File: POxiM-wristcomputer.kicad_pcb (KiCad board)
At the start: 4 copper layers, 40 x 23.5 mm, 82 parts, among them J1 USB_B_Micro, J14 Jumper_NO_Small, J2 AudioJack4_Ground

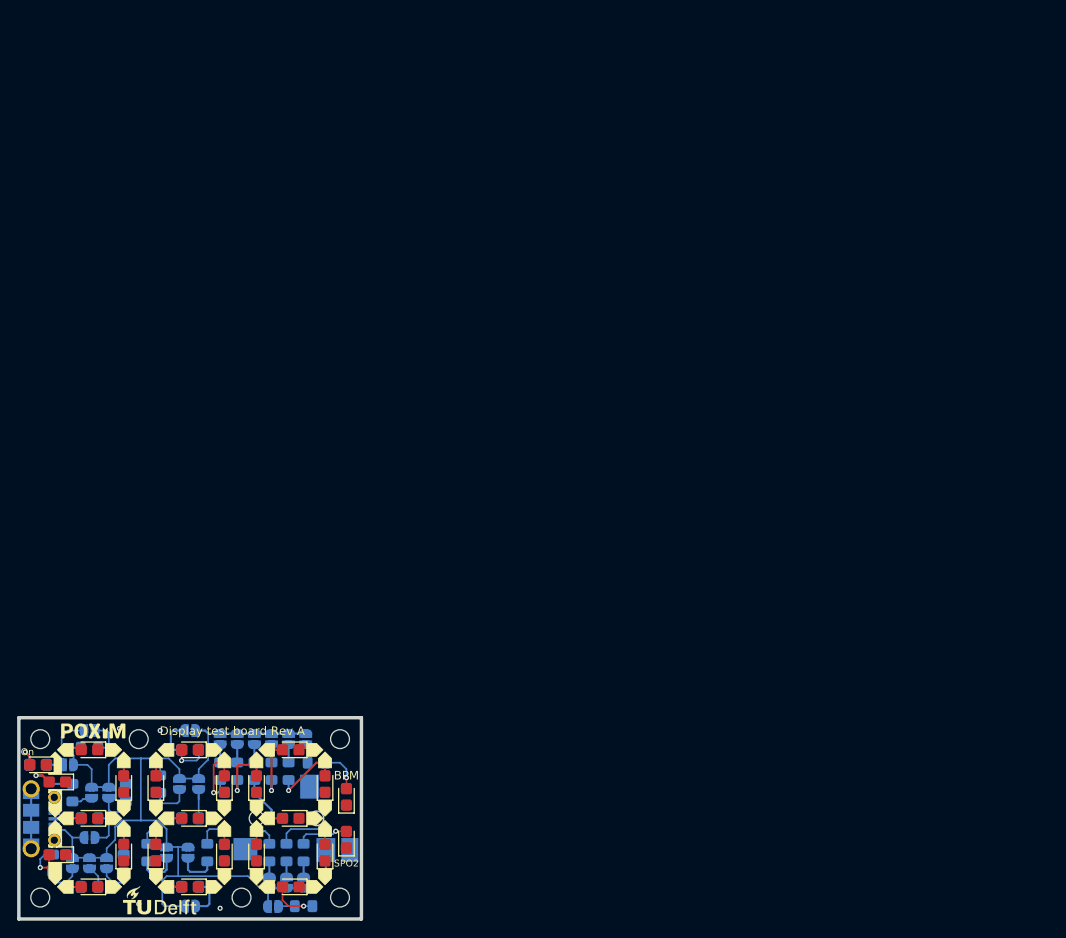
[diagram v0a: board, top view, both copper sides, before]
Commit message: Finish works-as prototype design
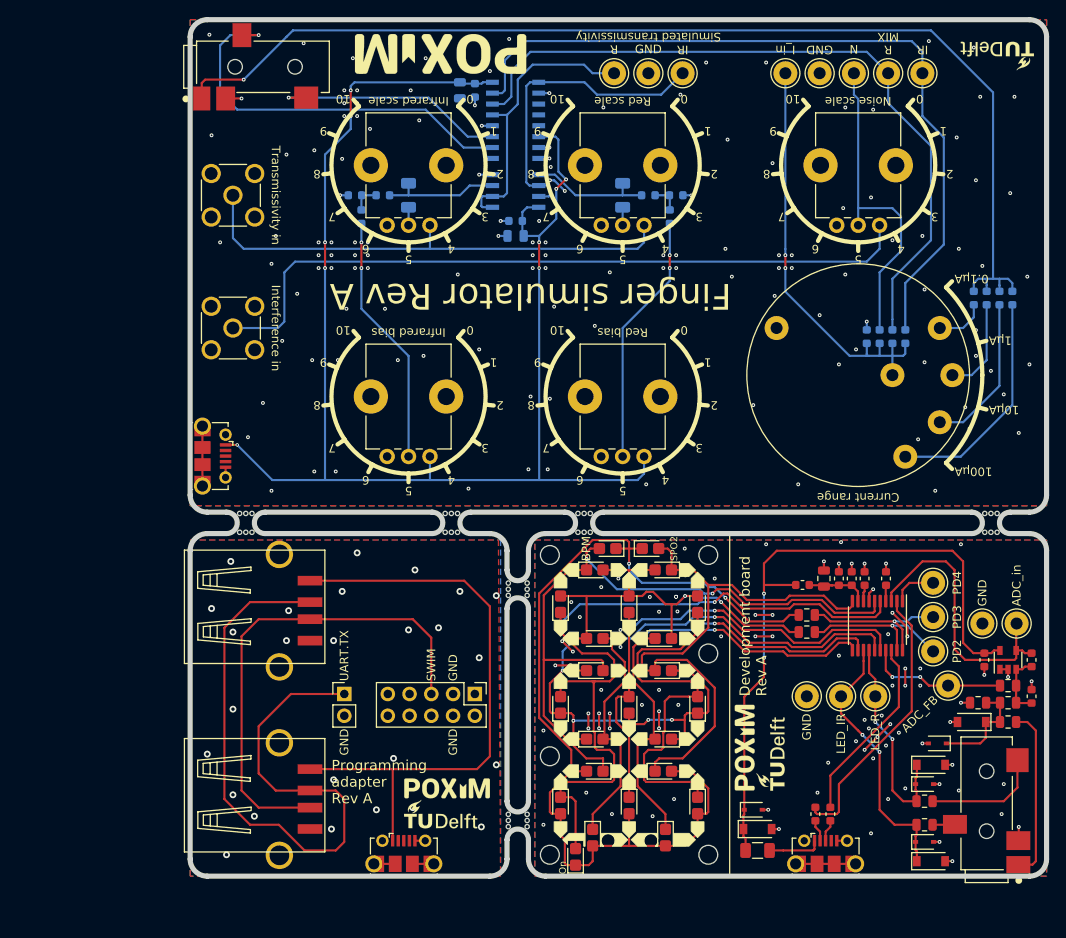
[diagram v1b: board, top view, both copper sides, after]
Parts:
- removed the G*** at (86.4, 142.8)
- removed the G*** at (78.7, 123.0)
- removed J14, JP16, JP18, JP20, JP27, JP28, JP29, JP30, JP31, JP8: Jumper_NO_Small, POxiM-uncategorised:SolderJumper-2_P1.3mm_Open_RoundedPad1.0x1.5mm
- removed JP10, JP11, JP12, JP13, JP15, JP17, JP19, JP21, JP22, JP23, JP24, JP25, JP26, JP9: Jumper_NC_Small, POxiM-uncategorised:SolderJumper-2_P1.3mm_SolderBridged_RoundedPad1.0x1.5mm
- removed R20, R21, R22, R23, R24, R25, R26, R27, R28, R29, R30: 4.7kΩ, Resistor_SMD:R_0805_2012Metric_Pad1.15x1.40mm_HandSolder
- added C1: 100nF, Capacitor_SMD:C_0603_1608Metric, F.Cu at (182.7, 114.8)
- added C10: 2.2uF, Capacitor_SMD:C_0805_2012Metric, B.Cu at (128.0, 65.2)
- added C11: 100nF, Capacitor_SMD:C_0603_1608Metric, B.Cu at (128.0, 63.5)
- added C12: 100nF, Capacitor_SMD:C_0603_1608Metric, B.Cu at (123.2, 48.2)
- added C13: 2.2uF, Capacitor_SMD:C_0805_2012Metric, B.Cu at (121.5, 48.2)
- added C14: 6.8uF, Capacitor_SMD:C_1206_3216Metric, B.Cu at (115.5, 60.5)
- added C15: 6.8uF, Capacitor_SMD:C_1206_3216Metric, B.Cu at (140.5, 60.5)
- added C16: 100nF, Capacitor_SMD:C_0603_1608Metric, B.Cu at (109.2, 60.5)
- added C17: 100nF, Capacitor_SMD:C_0603_1608Metric, B.Cu at (146.8, 60.5)
- added C2: 100pF, Capacitor_SMD:C_0603_1608Metric, F.Cu at (188.2, 114.8)
- added C3: 100nF, Capacitor_SMD:C_0603_1608Metric, F.Cu at (188.2, 119.0)
- added C4: 2.2uF, Capacitor_SMD:C_0805_2012Metric, F.Cu at (182.0, 119.8)
- added C5: 100nF, Capacitor_SMD:C_0603_1608Metric, F.Cu at (171.2, 105.2)
- added C6: 2.2uF, Capacitor_SMD:C_0805_2012Metric, F.Cu at (164.0, 105.2)
- added C7: 470nF, Capacitor_SMD:C_0603_1608Metric, F.Cu at (168.8, 105.2)
- added C8: 100nF, Capacitor_SMD:C_0603_1608Metric, F.Cu at (165.8, 105.2)
- added C9: 100nF, Capacitor_SMD:C_0603_1608Metric, F.Cu at (167.2, 105.2)
- added D1: 5.2V, Diode_SMD:D_SOD-123, F.Cu at (176.5, 138.2)
- added D2: ~, Diode_SMD:D_SOD-323, F.Cu at (175.8, 136.0)
- added D3: 5.2V, Diode_SMD:D_SOD-123, F.Cu at (176.5, 127.0)
- added D31: 5.2V, Diode_SMD:D_SOD-123, F.Cu at (156.2, 134.5)
- added D32: ~, Diode_SMD:D_SOD-323, F.Cu at (155.8, 132.2)
- added D4: ~, Diode_SMD:D_SOD-323, F.Cu at (175.8, 129.2)
- added D5: 5.2V, Diode_SMD:D_SOD-123, F.Cu at (181.2, 122.0)
- added D6: ~, Diode_SMD:D_SOD-323, F.Cu at (177.2, 124.5)
- added F1: 100mA, Resistor_SMD:R_1206_3216Metric, F.Cu at (156.2, 137.0)
- added FB1: Ferrite_Bead_Small, Inductor_SMD:L_0603_1608Metric, F.Cu at (161.5, 106.0)
- added G***: LOGO, POxiM-logos:POxiMLogo_GoldHeart_W10mm, F.Cu at (120.0, 129.8)
- added G***: LOGO, POxiM-logos:TUDelftLogo_W10mm, F.Cu at (119.2, 132.8)
- added G***: LOGO, POxiM-logos:TUDelftLogo_W10mm, F.Cu at (157.8, 125.8)
- added G***: LOGO, POxiM-logos:POxiMLogo_GoldHeart_W10mm, F.Cu at (154.8, 125.0)
- added G***: LOGO, POxiM-logos:TUDelftLogo_W10mm, F.Cu at (184.2, 44.2)
- added G***: LOGO, POxiM-logos:POxiMLogo_GoldHeart_W20mm, F.Cu at (119.2, 44.0)
- added J10: Transmissivity in, Connector_Coaxial:SMA_Molex_73251-2200_Horizontal, F.Cu at (95.0, 60.5)
- added J11: AudioJack4_Ground, POxiM-uncategorised:CUI_SJ-43514-SMT, F.Cu at (98.5, 45.5)
- added J3: USB_B_Micro, POxiM-uncategorised:Micro-B_Molex_105017-0001, F.Cu at (115.0, 140.0)
- added J4: USB_A, POxiM-uncategorised:USBA_87583-2010RLF, F.Cu at (104.0, 131.0)
- added J5: USB_A, POxiM-uncategorised:USBA_87583-2010RLF, F.Cu at (104.0, 109.0)
- added J6: Uart Out, Connector_PinHeader_2.54mm:PinHeader_1x02_P2.54mm_Vertical, F.Cu at (108.0, 118.7)
- added J7: Programming Header, Connector_PinHeader_2.54mm:PinHeader_2x05_P2.54mm_Vertical, F.Cu at (123.2, 118.7)
- added J8: USB_B_Micro, POxiM-uncategorised:Micro-B_Molex_105017-0001, F.Cu at (90.0, 91.0)
- added J9: Interference in, Connector_Coaxial:SMA_Molex_73251-2200_Horizontal, F.Cu at (95.0, 76.0)
- added JP1: Jumper_2_Open, Resistor_SMD:R_0603_1608Metric, F.Cu at (164.8, 132.8)
- added JP2: Jumper_2_Open, Resistor_SMD:R_0603_1608Metric, F.Cu at (163.0, 132.8)
- added MB1: Bumpon, POxiM-uncategorised:Bumpon-SJ-5007BK, B.Cu at (96.0, 131.0)
- added MB10: Bumpon, POxiM-uncategorised:Bumpon-SJ-5007BK, B.Cu at (184.0, 46.0)
- added MB11: Bumpon, POxiM-uncategorised:Bumpon-SJ-5007BK, B.Cu at (184.0, 91.5)
- added MB12: Bumpon, POxiM-uncategorised:Bumpon-SJ-5007BK, B.Cu at (96.0, 91.5)
- added MB2: Bumpon, POxiM-uncategorised:Bumpon-SJ-5007BK, B.Cu at (96.0, 109.0)
- added MB3: Bumpon, POxiM-uncategorised:Bumpon-SJ-5007BK, B.Cu at (121.0, 106.0)
- added MB4: Bumpon, POxiM-uncategorised:Bumpon-SJ-5007BK, B.Cu at (121.0, 134.0)
- added MB5: Bumpon, POxiM-uncategorised:Bumpon-SJ-5007BK, B.Cu at (139.5, 134.2)
- added MB6: Bumpon, POxiM-uncategorised:Bumpon-SJ-5007BK, B.Cu at (139.5, 105.8)
- added MB7: Bumpon, POxiM-uncategorised:Bumpon-SJ-5007BK, B.Cu at (184.0, 134.0)
- added MB8: Bumpon, POxiM-uncategorised:Bumpon-SJ-5007BK, B.Cu at (184.0, 106.0)
- added MB9: Bumpon, POxiM-uncategorised:Bumpon-SJ-5007BK, B.Cu at (96.0, 46.0)
- added R1: 3.3MΩ, Resistor_SMD:R_0805_2012Metric, F.Cu at (185.5, 117.8)
- added R2: 1k, Resistor_SMD:R_0805_2012Metric, F.Cu at (185.5, 119.8)
- added R3: 100, Resistor_SMD:R_0805_2012Metric, F.Cu at (185.5, 122.0)
- added R4: 100, Resistor_SMD:R_0805_2012Metric, F.Cu at (175.8, 131.2)
- added R5: 100, Resistor_SMD:R_0805_2012Metric, F.Cu at (175.8, 134.0)
- added R6: R_Small, Resistor_SMD:R_0805_2012Metric, F.Cu at (162.0, 111.5)
- added RV1: 1k, POxiM-uncategorised:Potentiometer_Bourns_PTV09A-1_Single_Vertical, F.Cu at (170.5, 64.0)
- added RV2: 1k, POxiM-uncategorised:Potentiometer_Bourns_PTV09A-1_Single_Vertical, F.Cu at (118.0, 64.0)
- added RV3: 1k, POxiM-uncategorised:Potentiometer_Bourns_PTV09A-1_Single_Vertical, F.Cu at (118.0, 91.0)
- added RV4: 1k, POxiM-uncategorised:Potentiometer_Bourns_PTV09A-1_Single_Vertical, F.Cu at (143.0, 64.0)
- added RV5: 1k, POxiM-uncategorised:Potentiometer_Bourns_PTV09A-1_Single_Vertical, F.Cu at (143.0, 91.0)
- added SW1: Current range, POxiM-uncategorised:SW_ESwitch_KC14A10.001NPS, F.Cu at (168.0, 81.5)
- added TP1: LED_IR, TestPoint:TestPoint_Loop_D2.60mm_Drill1.4mm_Beaded, F.Cu at (166.0, 119.0)
- added TP10: IR, TestPoint:TestPoint_Loop_D2.60mm_Drill1.4mm_Beaded, F.Cu at (147.5, 46.2)
- added TP11: R, TestPoint:TestPoint_Loop_D2.60mm_Drill1.4mm_Beaded, F.Cu at (171.5, 46.2)
- added TP12: IR, TestPoint:TestPoint_Loop_D2.60mm_Drill1.4mm_Beaded, F.Cu at (175.5, 46.2)
- added TP13: I_in, TestPoint:TestPoint_Loop_D2.60mm_Drill1.4mm_Beaded, F.Cu at (159.5, 46.2)
- added TP16: N, TestPoint:TestPoint_Loop_D2.60mm_Drill1.4mm_Beaded, F.Cu at (167.5, 46.2)
- added TP17: R, TestPoint:TestPoint_Loop_D2.60mm_Drill1.4mm_Beaded, F.Cu at (139.5, 46.2)
- added TP19: GND, TestPoint:TestPoint_Loop_D2.60mm_Drill1.4mm_Beaded, F.Cu at (162.0, 119.0)
- added TP2: LED_R, TestPoint:TestPoint_Loop_D2.60mm_Drill1.4mm_Beaded, F.Cu at (170.0, 119.0)
- added TP20: GND, TestPoint:TestPoint_Loop_D2.60mm_Drill1.4mm_Beaded, F.Cu at (182.5, 110.5)
- added TP3: ADC_FB, TestPoint:TestPoint_Loop_D2.60mm_Drill1.4mm_Beaded, F.Cu at (178.5, 117.8)
- added TP4: ADC_in, TestPoint:TestPoint_Loop_D2.60mm_Drill1.4mm_Beaded, F.Cu at (186.5, 110.5)
- added TP5: PD3, TestPoint:TestPoint_Loop_D2.60mm_Drill1.4mm_Beaded, F.Cu at (176.8, 109.8)
- added TP6: PD4, TestPoint:TestPoint_Loop_D2.60mm_Drill1.4mm_Beaded, F.Cu at (176.8, 105.8)
- added TP7: PD2, TestPoint:TestPoint_Loop_D2.60mm_Drill1.4mm_Beaded, F.Cu at (176.8, 113.8)
- added TP8: GND, TestPoint:TestPoint_Loop_D2.60mm_Drill1.4mm_Beaded, F.Cu at (143.5, 46.2)
- added TP9: GND, TestPoint:TestPoint_Loop_D2.60mm_Drill1.4mm_Beaded, F.Cu at (163.5, 46.2)
- added U1: LM321, Package_TO_SOT_SMD:SOT-23-5, F.Cu at (185.5, 114.8)
- added U2: STM8S003F3P, Package_SO:TSSOP-20_4.4x6.5mm_P0.65mm, F.Cu at (170.2, 110.8)
- added U3: LM358, Package_SO:SOIC-8_3.9x4.9mm_P1.27mm, B.Cu at (128.0, 60.0)
- added U4: NLAS4053, Package_SO:SOIC-16_3.9x9.9mm_P1.27mm, B.Cu at (128.0, 51.8)
- added mouse-bite-2.54mm-slot: VAL**, Panelization:mouse-bite-2.5mm-slot, F.Cu at (96.5, 98.8)
- added mouse-bite-2.54mm-slot: VAL**, Panelization:mouse-bite-2.5mm-slot, F.Cu at (128.2, 133.5)
- added mouse-bite-2.54mm-slot: VAL**, Panelization:mouse-bite-2.5mm-slot, F.Cu at (128.2, 106.5)
- added mouse-bite-2.54mm-slot: VAL**, Panelization:mouse-bite-2.5mm-slot, F.Cu at (120.5, 98.8)
- added mouse-bite-2.54mm-slot: VAL**, Panelization:mouse-bite-2.5mm-slot, F.Cu at (136.0, 98.8)
- added mouse-bite-2.54mm-slot: VAL**, Panelization:mouse-bite-2.5mm-slot, F.Cu at (183.5, 98.8)
- J1, J2: moved to F.Cu
- R10, R18, R19, R8, R9: value 4.7kΩ -> 27kΩ; footprint Resistor_SMD:R_0805_2012Metric_Pad1.15x1.40mm_HandSolder -> Resistor_SMD:R_0603_1608Metric
- R11: value 4.7kΩ -> 1kΩ; footprint Resistor_SMD:R_0805_2012Metric_Pad1.15x1.40mm_HandSolder -> Resistor_SMD:R_0603_1608Metric
- R12: value 4.7kΩ -> 4.7MΩ; footprint Resistor_SMD:R_0805_2012Metric_Pad1.15x1.40mm_HandSolder -> Resistor_SMD:R_0603_1608Metric
- R13: value 4.7kΩ -> 470kΩ; footprint Resistor_SMD:R_0805_2012Metric_Pad1.15x1.40mm_HandSolder -> Resistor_SMD:R_0603_1608Metric
- R14: value 4.7kΩ -> 47kΩ; footprint Resistor_SMD:R_0805_2012Metric_Pad1.15x1.40mm_HandSolder -> Resistor_SMD:R_0603_1608Metric
- R15: footprint Resistor_SMD:R_0805_2012Metric_Pad1.15x1.40mm_HandSolder -> Resistor_SMD:R_0603_1608Metric
- R16, R17: value 4.7kΩ -> 510k; footprint Resistor_SMD:R_0805_2012Metric_Pad1.15x1.40mm_HandSolder -> Resistor_SMD:R_0603_1608Metric
- R7: value 4.7kΩ -> R_Small; footprint Resistor_SMD:R_0805_2012Metric_Pad1.15x1.40mm_HandSolder -> Resistor_SMD:R_0805_2012Metric; moved to F.Cu
- moved R14 126.6 mm to (184.5, 72.5), turned to 270 degrees
- moved R12 119.2 mm to (181.5, 72.5), turned to 270 degrees
- moved R15 108.3 mm to (186.0, 72.5), turned to 270 degrees
- moved R13 106.8 mm to (183.0, 72.5), turned to 270 degrees
- moved R8 106.7 mm to (173.5, 77.0), turned to 90 degrees
- moved R10 102.9 mm to (170.5, 77.0)
- moved J1 94.5 mm to (164.2, 140.0), turned to 0 degrees
- moved R11 90.7 mm to (169.0, 77.0), turned to 270 degrees
- moved R16 87.0 mm to (112.5, 60.5), turned to 180 degrees
- moved R9 86.9 mm to (172.0, 77.0), turned to 90 degrees
- moved R17 82.6 mm to (143.5, 60.5), turned to 0 degrees
- moved J2 81.5 mm to (183.0, 131.5), turned to 90 degrees
- moved R19 80.9 mm to (146.0, 63.0)
- moved H4 78.2 mm to (150.5, 137.5), turned to 90 degrees
- moved R18 75.2 mm to (110.0, 63.0), turned to 270 degrees
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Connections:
- D10 pad 1: GND -> /Display/Segment1
- D11 pad 1: GND -> /Display/Segment2
- D12 pad 1: GND -> /Display/Segment2
- D12 pad 2: Net-(D12-Pad2) -> Net-(D10-Pad2)
- D13 pad 1: GND -> /Display/Segment3
- D13 pad 2: Net-(D13-Pad2) -> Net-(D11-Pad2)
- D14 pad 1: GND -> /Display/Segment3
- D14 pad 2: Net-(D14-Pad2) -> Net-(D10-Pad2)
- D15 pad 1: GND -> /Display/Segment4
- D15 pad 2: Net-(D15-Pad2) -> Net-(D11-Pad2)
- D16 pad 1: GND -> /Display/Segment4
- D16 pad 2: Net-(D16-Pad2) -> Net-(D10-Pad2)
- D17 pad 1: GND -> /Display/Segment5
- D17 pad 2: Net-(D17-Pad2) -> Net-(D11-Pad2)
- D18 pad 1: GND -> /Display/Segment5
- D18 pad 2: Net-(D18-Pad2) -> Net-(D10-Pad2)
- D19 pad 1: GND -> /Display/Segment6
- D19 pad 2: Net-(D19-Pad2) -> Net-(D11-Pad2)
- D20 pad 1: GND -> /Display/Segment6
- D20 pad 2: Net-(D20-Pad2) -> Net-(D10-Pad2)
- D21 pad 1: GND -> Net-(D11-Pad2)
- D21 pad 2: Net-(D21-Pad2) -> /Display/Segment0
- D22 pad 1: GND -> Net-(D10-Pad2)
- D22 pad 2: Net-(D22-Pad2) -> /Display/Segment0
- D23 pad 1: GND -> Net-(D11-Pad2)
- D23 pad 2: Net-(D23-Pad2) -> /Display/Segment1
- D24 pad 1: GND -> Net-(D10-Pad2)
- D24 pad 2: Net-(D24-Pad2) -> /Display/Segment1
- D25 pad 1: GND -> Net-(D11-Pad2)
- D25 pad 2: Net-(D25-Pad2) -> /Display/Segment2
- D26 pad 1: GND -> Net-(D10-Pad2)
- D26 pad 2: Net-(D26-Pad2) -> /Display/Segment2
- D27 pad 1: GND -> Net-(D11-Pad2)
- D27 pad 2: Net-(D27-Pad2) -> /Display/Segment3
- D28 pad 1: GND -> Net-(D11-Pad2)
- D28 pad 2: Net-(D28-Pad2) -> /Display/Segment4
- D29 pad 1: GND -> Net-(D11-Pad2)
- D29 pad 2: Net-(D29-Pad2) -> /Display/Segment5
- D30 pad 1: GND -> Net-(D11-Pad2)
- D30 pad 2: Net-(D30-Pad2) -> /Display/Segment6
- D7 pad 1: GND -> /Display/Segment0
- D7 pad 2: Net-(D7-Pad2) -> Net-(D11-Pad2)
- D8 pad 1: GND -> /Display/Segment0
- D8 pad 2: Net-(D8-Pad2) -> Net-(D10-Pad2)
- D9 pad 1: GND -> /Display/Segment1
- D9 pad 2: Net-(D9-Pad2) -> Net-(D11-Pad2)
- J1 pad 1: +5V -> /5V_power_input
- J1 pad 2: Net-(J1-Pad2) -> /USB interface/Data-
- J1 pad 3: Net-(J1-Pad3) -> /USB interface/Data+
- J2 pad R1: Net-(J2-PadR1) -> /Signal conditioning/LEDOut.IR
- J2 pad S: Net-(J2-PadS) -> /Signal conditioning/PhotoDiode
- J2 pad T: Net-(J2-PadT) -> /Signal conditioning/LEDOut.Red
- R10 pad 1: Net-(JP11-Pad2) -> Net-(R10-Pad1)
- R10 pad 2: Net-(D10-Pad2) -> Net-(R10-Pad2)
- R11 pad 1: Net-(JP12-Pad2) -> /Testing finger board/GND
- R11 pad 2: Net-(D11-Pad2) -> Net-(R10-Pad1)
- R12 pad 1: Net-(JP13-Pad2) -> /Testing finger board/Photodiode
- R12 pad 2: Net-(D12-Pad2) -> Net-(R12-Pad2)
- R13 pad 1: Net-(J14-Pad2) -> /Testing finger board/Photodiode
- R13 pad 2: Net-(D13-Pad2) -> Net-(R13-Pad2)
- R14 pad 1: Net-(JP15-Pad2) -> /Testing finger board/Photodiode
- R14 pad 2: Net-(D14-Pad2) -> Net-(R14-Pad2)
- R15 pad 1: Net-(JP16-Pad2) -> /Testing finger board/Photodiode
- R15 pad 2: Net-(D15-Pad2) -> Net-(R15-Pad2)
- R16 pad 1: Net-(JP17-Pad2) -> /Testing finger board/heartbeat bias and scaling RED/Out
- R16 pad 2: Net-(D16-Pad2) -> Net-(C16-Pad1)
- R17 pad 1: Net-(JP18-Pad2) -> /Testing finger board/heartbeat bias and scaling IR/Out
- R17 pad 2: Net-(D17-Pad2) -> Net-(C17-Pad1)
- R18 pad 1: Net-(JP19-Pad2) -> Net-(C16-Pad1)
- R18 pad 2: Net-(D18-Pad2) -> Net-(R18-Pad2)
- R19 pad 1: Net-(JP20-Pad2) -> Net-(C17-Pad1)
- R19 pad 2: Net-(D19-Pad2) -> Net-(R19-Pad2)
- R7 pad 1: Net-(JP8-Pad2) -> /Display/Common1
- R7 pad 2: Net-(D7-Pad2) -> Net-(D10-Pad2)
- R8 pad 1: Net-(JP9-Pad2) -> Net-(R10-Pad1)
- R8 pad 2: Net-(D8-Pad2) -> Net-(R8-Pad2)
- R9 pad 1: Net-(JP10-Pad2) -> Net-(R10-Pad1)
- R9 pad 2: Net-(D9-Pad2) -> Net-(R9-Pad2)
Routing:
- net /Testing finger board/5V: track 0.00 -> 170.6 mm, vias 0 -> 9
- net /Testing finger board/Photodiode: track 0.00 -> 131.3 mm, vias 0 -> 1
- net Net-(D10-Pad2): track 3.62 -> 112.8 mm, vias 1 -> 2
- net Net-(D11-Pad2): track 7.72 -> 100.5 mm, vias 1 -> 8
- net Net-(R8-Pad2): track 0.00 -> 91.6 mm
- net /Display/Segment0: track 0.00 -> 90.6 mm, vias 0 -> 2
- net Net-(R9-Pad2): track 0.00 -> 86.4 mm
- net /Testing finger board/Mains_noise: track 0.00 -> 85.4 mm
- net Net-(J4-Pad2): track 0.00 -> 81.4 mm
- net /Display/Segment1: track 0.00 -> 80.9 mm, vias 0 -> 2
- net Net-(J3-Pad1): track 0.00 -> 69.7 mm
- net /Display/Segment2: track 0.00 -> 68.7 mm
- net /Display/Segment3: track 0.00 -> 66.7 mm, vias 0 -> 2
- net /Display/Segment5: track 0.00 -> 63.5 mm, vias 0 -> 2
- net /Testing finger board/Heartbeat: track 0.00 -> 58.6 mm
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- added copper zone on B.Cu, net /Testing finger board/GND
- added copper zone on F.Cu, net /Testing finger board/GND
- added copper zone on B.Cu, net Net-(J3-Pad5)
- added copper zone on F.Cu, net Net-(J3-Pad5)
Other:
- board size 40 x 23.5 mm -> 100 x 100 mm
- board text added: "0"
- board text added: "0.1µA"
- board text added: "1"
- board text added: "10"
- board text added: "100µA"
- board text added: "10µA"
- board text added: "1µA"
- board text added: "2"
- board text added: "3"
- board text added: "4"
- board text added: "5"
- board text added: "6"
- board text added: "7"
- board text added: "8"
- board text added: "9"
- board text added: "Current range"
- board text added: "Development board Rev A"
- board text added: "Finger simulator Rev A"
- board text added: "GND"
- board text added: "Infrared bias"
- board text added: "Infrared scale"
- board text added: "MIX"
- board text added: "Noise scale"
- board text added: "Programming adapter Rev A"
- board text added: "Red bias"
- board text added: "Red scale"
- board text added: "SWIM"
- board text added: "Simulated transmissivity"
- board text added: "ToDo: - Run DRC - Add potentiometer knobs to BOM"
- board text added: "UART.TX"
- board text removed: "Display test board Rev A"

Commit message: Finalise works-like prototype
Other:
- copper layers 4 -> 2
- board text removed: "ToDo: - Run DRC - Add potentiometer knobs to BOM"
